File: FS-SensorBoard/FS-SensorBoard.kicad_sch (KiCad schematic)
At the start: 58 parts, among them J1 USB_B, J2 Conn_01x02_Pin, M1 MountingHole, M2 MountingHole, M3 MountingHole, M4 MountingHole, U1 CH340C, U2 ESP32-WROOM-32, U3 TJA1051TK-3, U4 LM2576S-3.3, U5 LM2576S-5

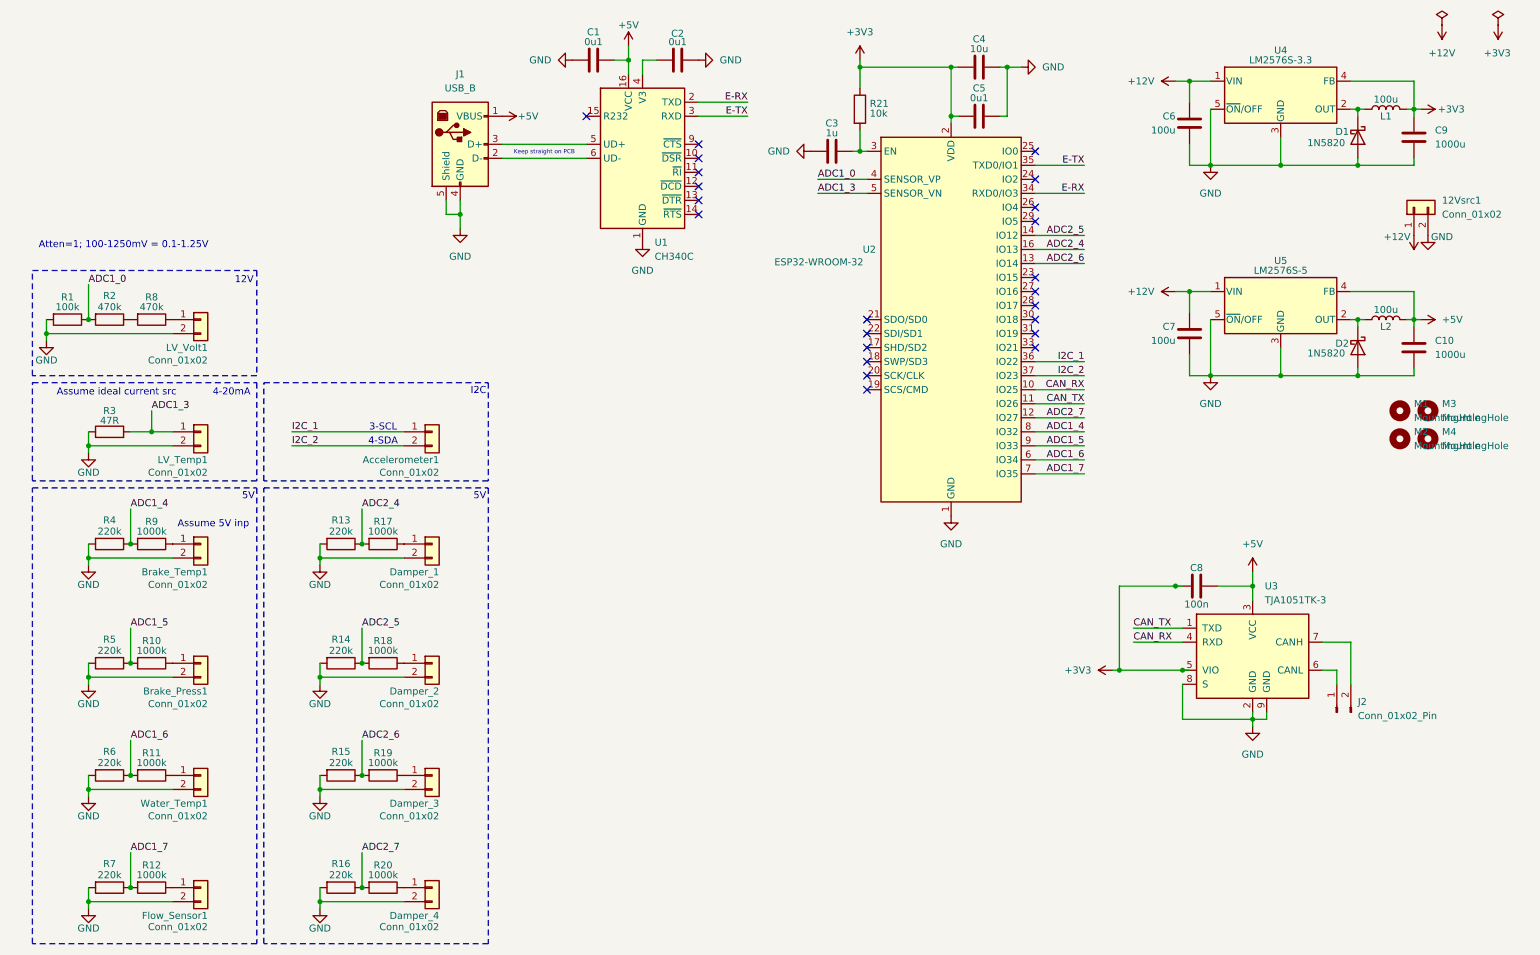
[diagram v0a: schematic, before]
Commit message: Version1
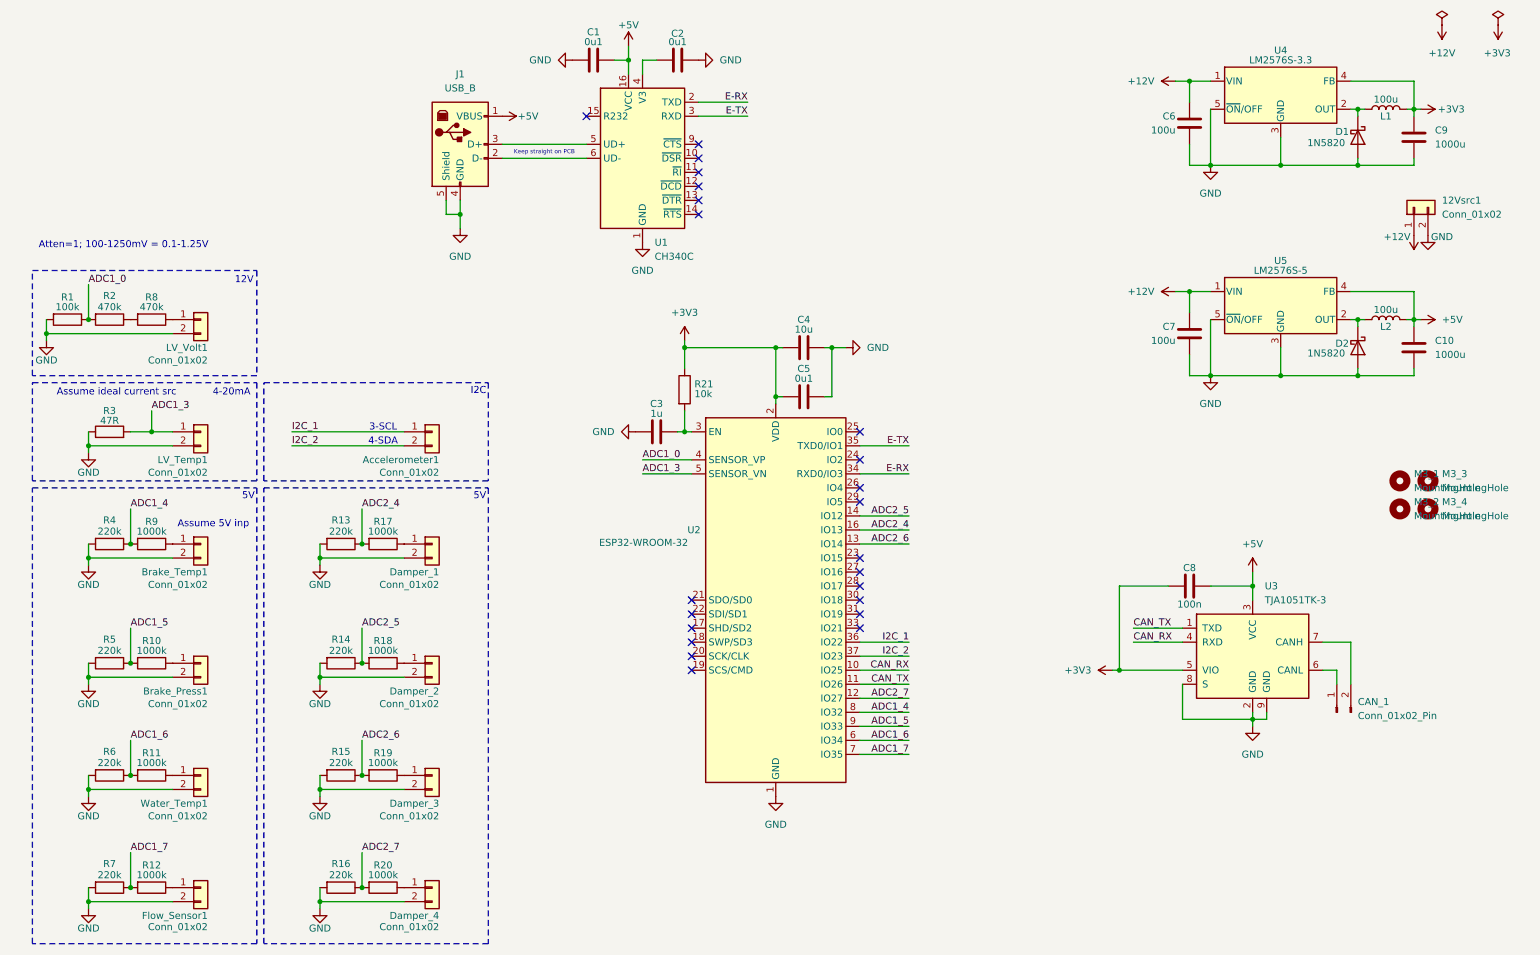
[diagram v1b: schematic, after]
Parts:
- renumbered J2 to CAN_1, M1 to M3_1, M2 to M3_2, M3 to M3_3, M4 to M3_4
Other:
- moved on the sheet: C3, C4, C5, C8, M3_1, M3_2, M3_3, M3_4, R21, U2
